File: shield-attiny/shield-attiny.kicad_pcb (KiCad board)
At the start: 2 copper layers, 68.9 x 53.6 mm, 9 parts, among them SW1 SW_Push, U1 ATtiny85-20PU

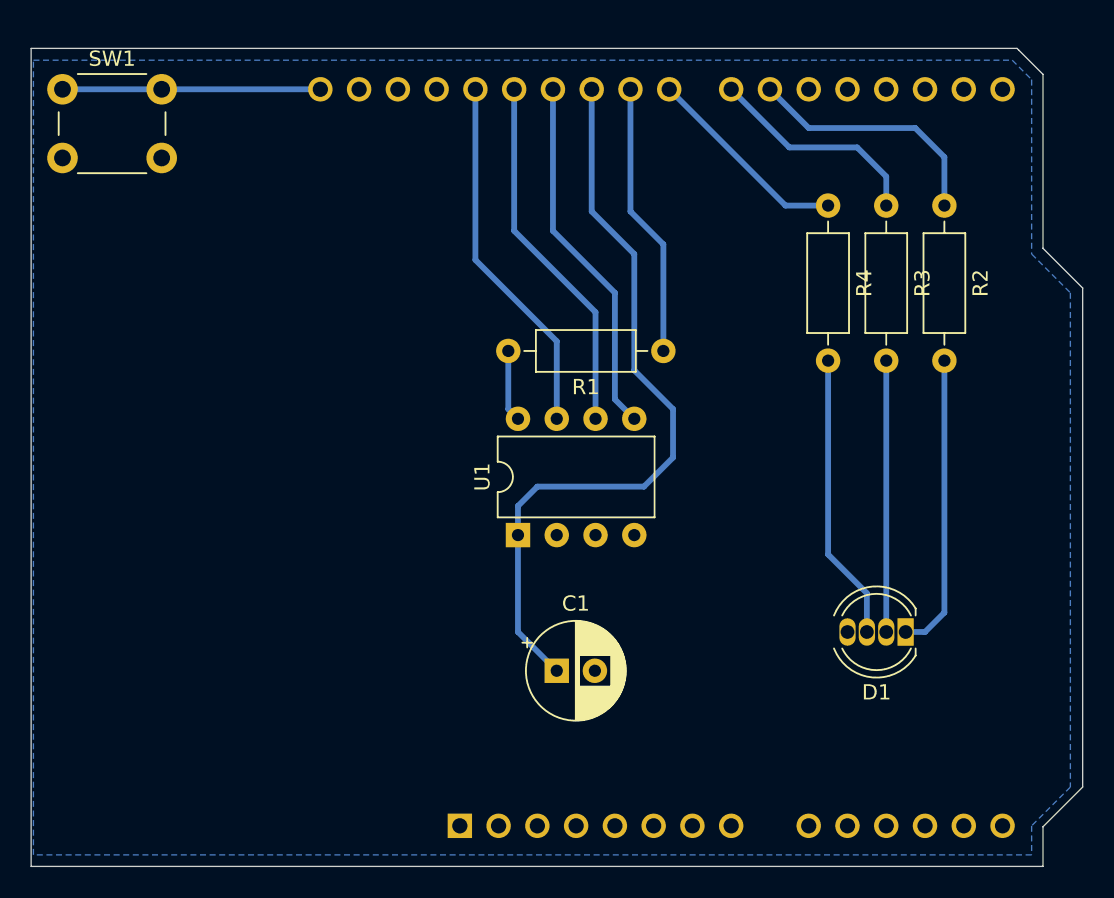
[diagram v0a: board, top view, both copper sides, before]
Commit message: Adiconando Layout
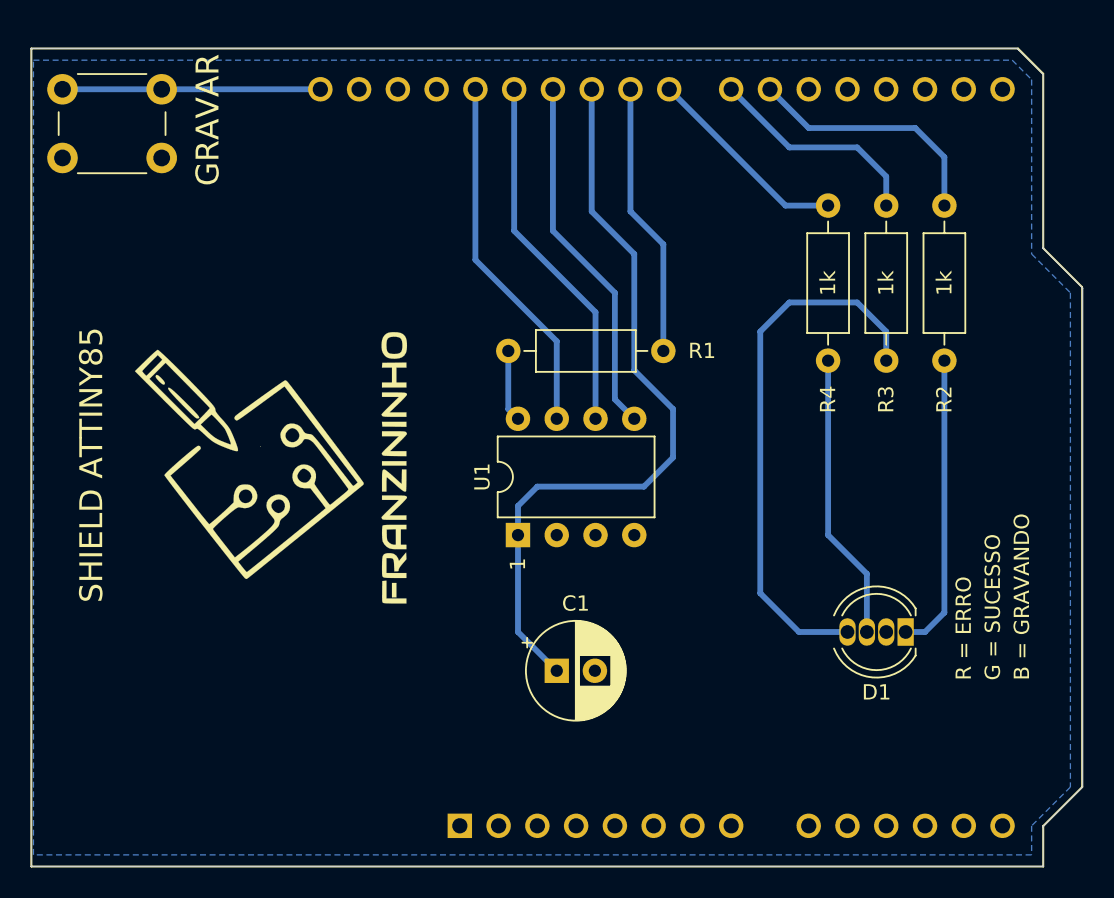
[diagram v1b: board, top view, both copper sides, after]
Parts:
- added G***: LOGO, graphics:logo, F.Cu at (123.8, 93.3)
- A1: footprint Module:Arduino_UNO_R3 -> shield-attiny:Shield_Arduino_UNO_R3; moved to F.Cu
- D1: value LED_RGBC -> LED_RCBG
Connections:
- D1 pad 2: Net-(D1-Pad2) -> GND
- D1 pad 4: GND -> Net-(D1-Pad4)
- R3 pad 2: Net-(D1-Pad2) -> Net-(D1-Pad4)
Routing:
- net Net-(D1-Pad4): track 0.00 -> 35.7 mm
- net Net-(D1-Pad2): track 17.8 -> 0.00 mm
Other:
- board text added: "1"
- board text added: "B = GRAVANDO"
- board text added: "G = SUCESSO"
- board text added: "GRAVAR"
- board text added: "R = ERRO"
- board text added: "SHIELD ATTINY85"
